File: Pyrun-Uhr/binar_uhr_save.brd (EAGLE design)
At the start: 100 x 50 mm, 64 parts, among them IC1 74HC595D, IC2 74HC595D

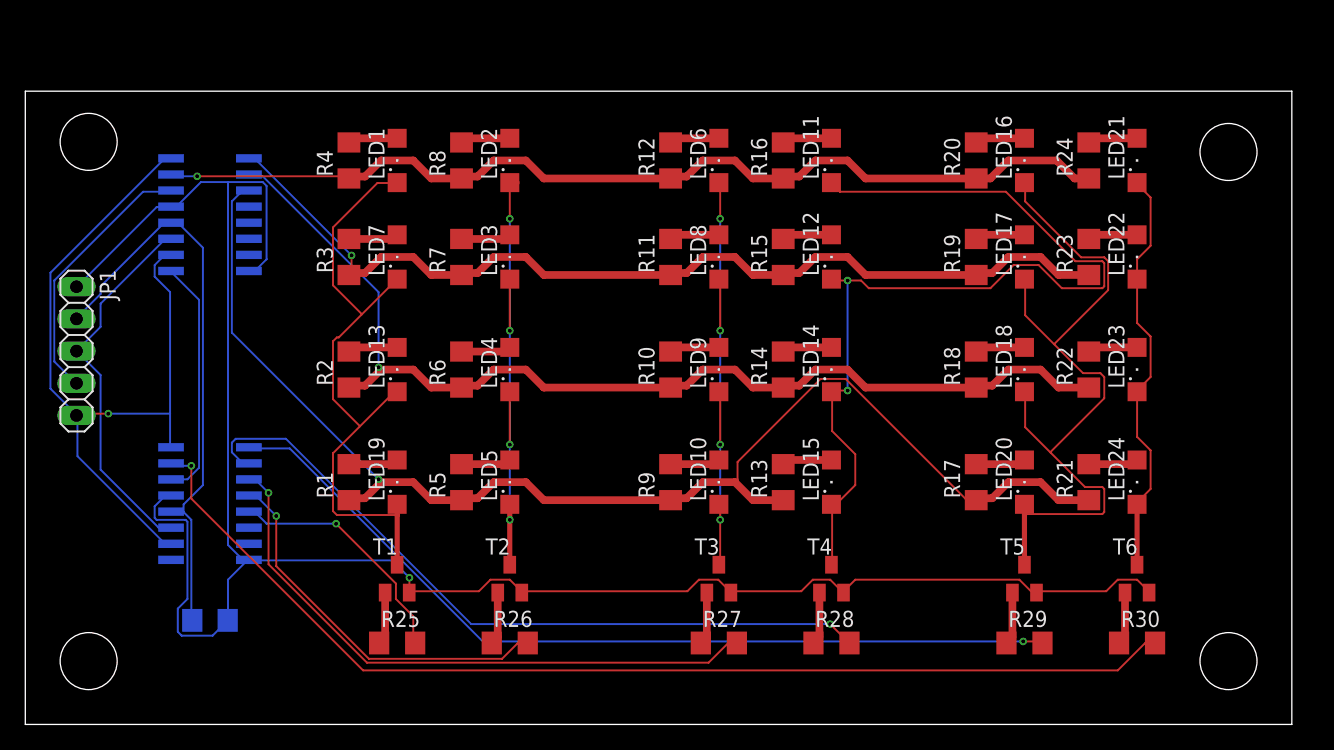
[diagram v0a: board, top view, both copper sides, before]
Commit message: smart home platine now v3
lets try it now
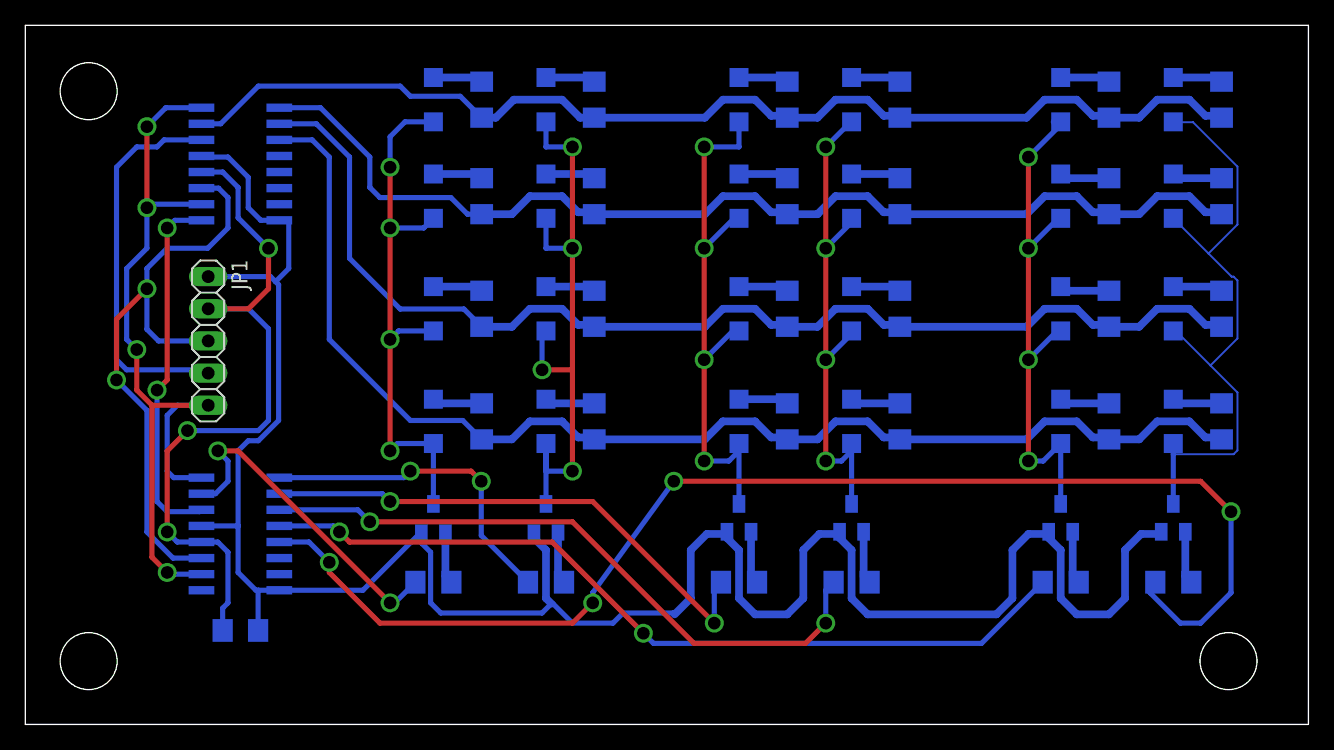
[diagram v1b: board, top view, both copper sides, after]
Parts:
- moved R1 69.1 mm to (94.5, 23.9), flipped to the bottom
- moved R2 69.1 mm to (94.5, 32.8), flipped to the bottom
- moved R3 69.1 mm to (94.5, 41.7), flipped to the bottom
- moved R4 69.1 mm to (94.5, 49.3), flipped to the bottom
- moved LED1 61.5 mm to (90.6, 49.3), flipped to the bottom
- moved LED13 61.5 mm to (90.6, 32.8), flipped to the bottom
- moved LED19 61.5 mm to (90.6, 23.9), flipped to the bottom
- moved LED7 61.5 mm to (90.6, 41.7), flipped to the bottom
- moved R25 61.5 mm to (90.6, 11.2), flipped to the bottom
- moved T1 61.5 mm to (90.6, 16.3), flipped to the bottom
- moved LED21 55.8 mm to (32.2, 49.3), flipped to the bottom
- moved LED22 55.8 mm to (32.2, 41.7), flipped to the bottom
- moved LED23 55.8 mm to (32.2, 32.8), flipped to the bottom
- moved LED24 55.8 mm to (32.2, 23.9), flipped to the bottom
- moved R30 55.8 mm to (32.2, 11.2), flipped to the bottom
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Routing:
- net LC1: track 19.3 -> 101.0 mm, vias 1 -> 4
- net LC6: track 86.9 -> 26.5 mm, vias 1 -> 2
- net LC5: track 69.1 -> 26.0 mm, vias 1 -> 2
- net LC2: track 30.2 -> 66.1 mm, vias 1 -> 2
- net N$52: track 75.0 -> 44.8 mm, vias 2 -> 4
- net SH_CP: track 29.8 -> 48.9 mm, vias 0 -> 2
- net GND: track 158.6 -> 175.9 mm, vias 1 -> 0
- net LC4: track 58.0 -> 42.0 mm, vias 1 -> 2
- net N$20: track 61.2 -> 48.9 mm, vias 0 -> 4
- net N$6: track 32.8 -> 44.6 mm, vias 0 -> 4
- net ST_CP: track 46.7 -> 57.7 mm, vias 0 -> 3
- net LR1: track 78.5 -> 88.7 mm, vias 1 -> 0
- net N$4: track 19.0 -> 28.8 mm, vias 0 -> 2
- net DS: track 21.0 -> 30.5 mm
- net LR2: track 77.2 -> 85.2 mm, vias 1 -> 0
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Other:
- board size 100 x 50 mm -> 101.3 x 55.2 mm
